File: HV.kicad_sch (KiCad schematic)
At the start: 15 parts, among them J401 1935161, J402 Header_Male_Pin_2.54mm_1X3_,_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, J403 RF1-01K-D-00-50-BK-HDW, J404 1935161, J405 RF1-01K-D-00-50-BK-HDW, Q401 MCB90N12A-TP, Q402 MCB90N12A-TP, U401 TMCS1108A4UQDR

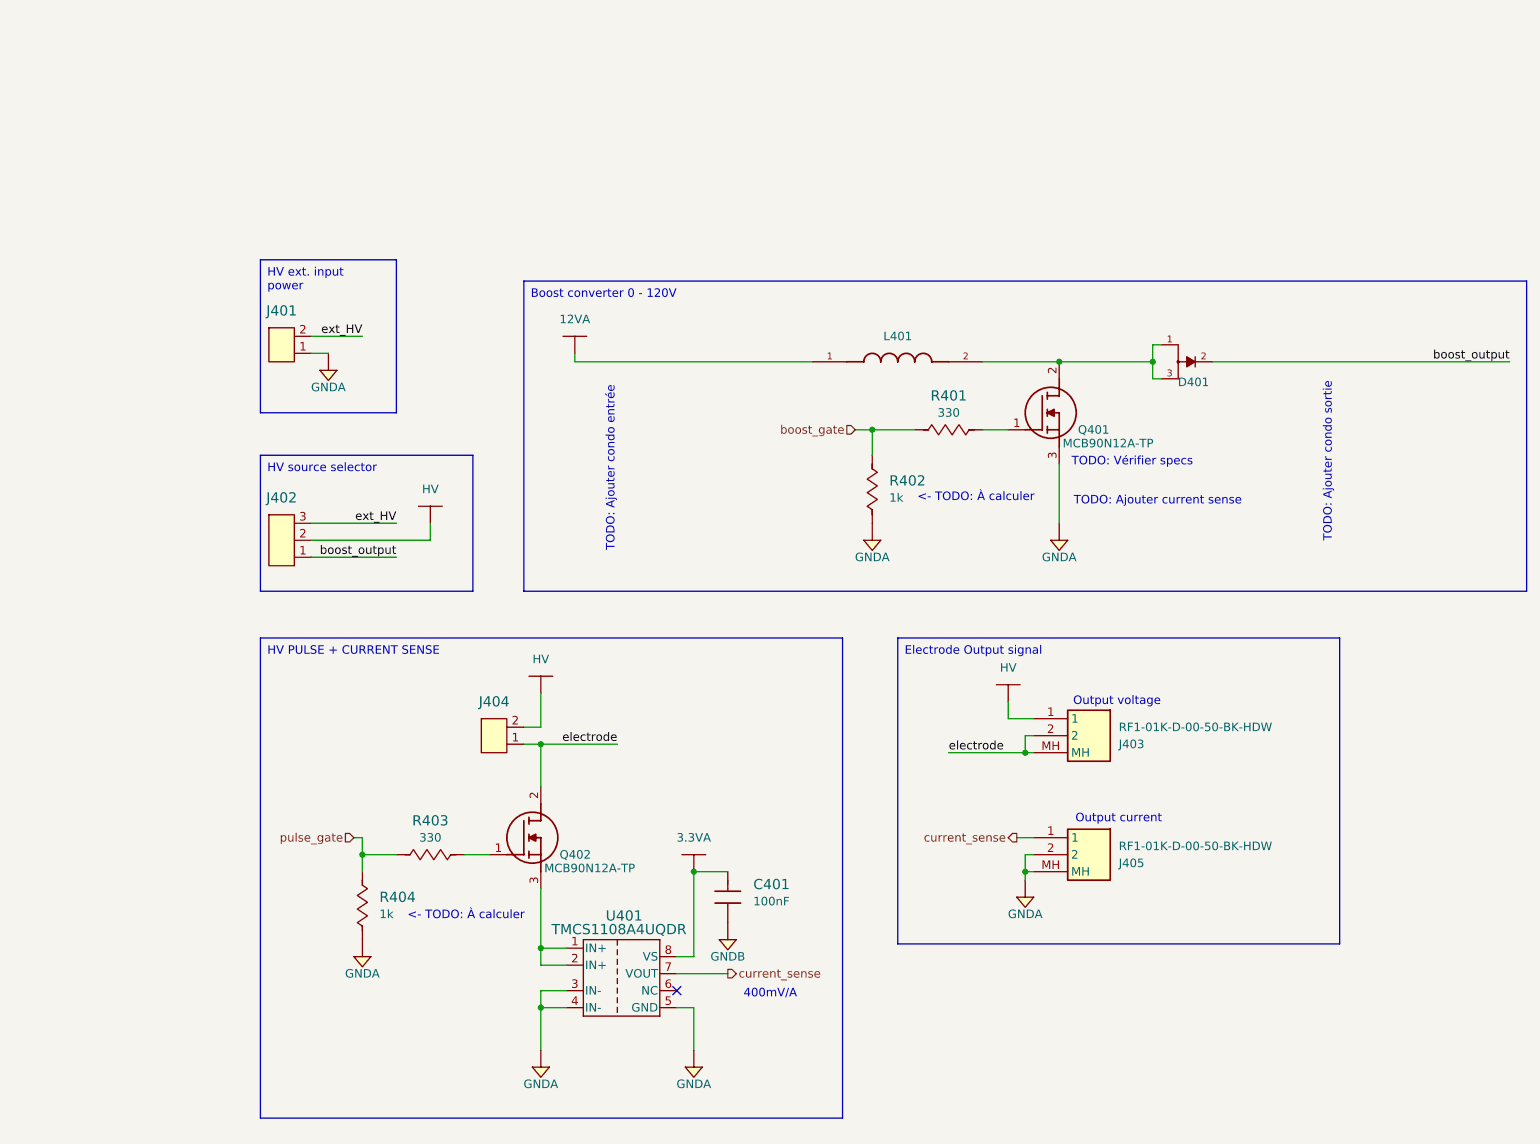
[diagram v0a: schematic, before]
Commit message: modif schématique
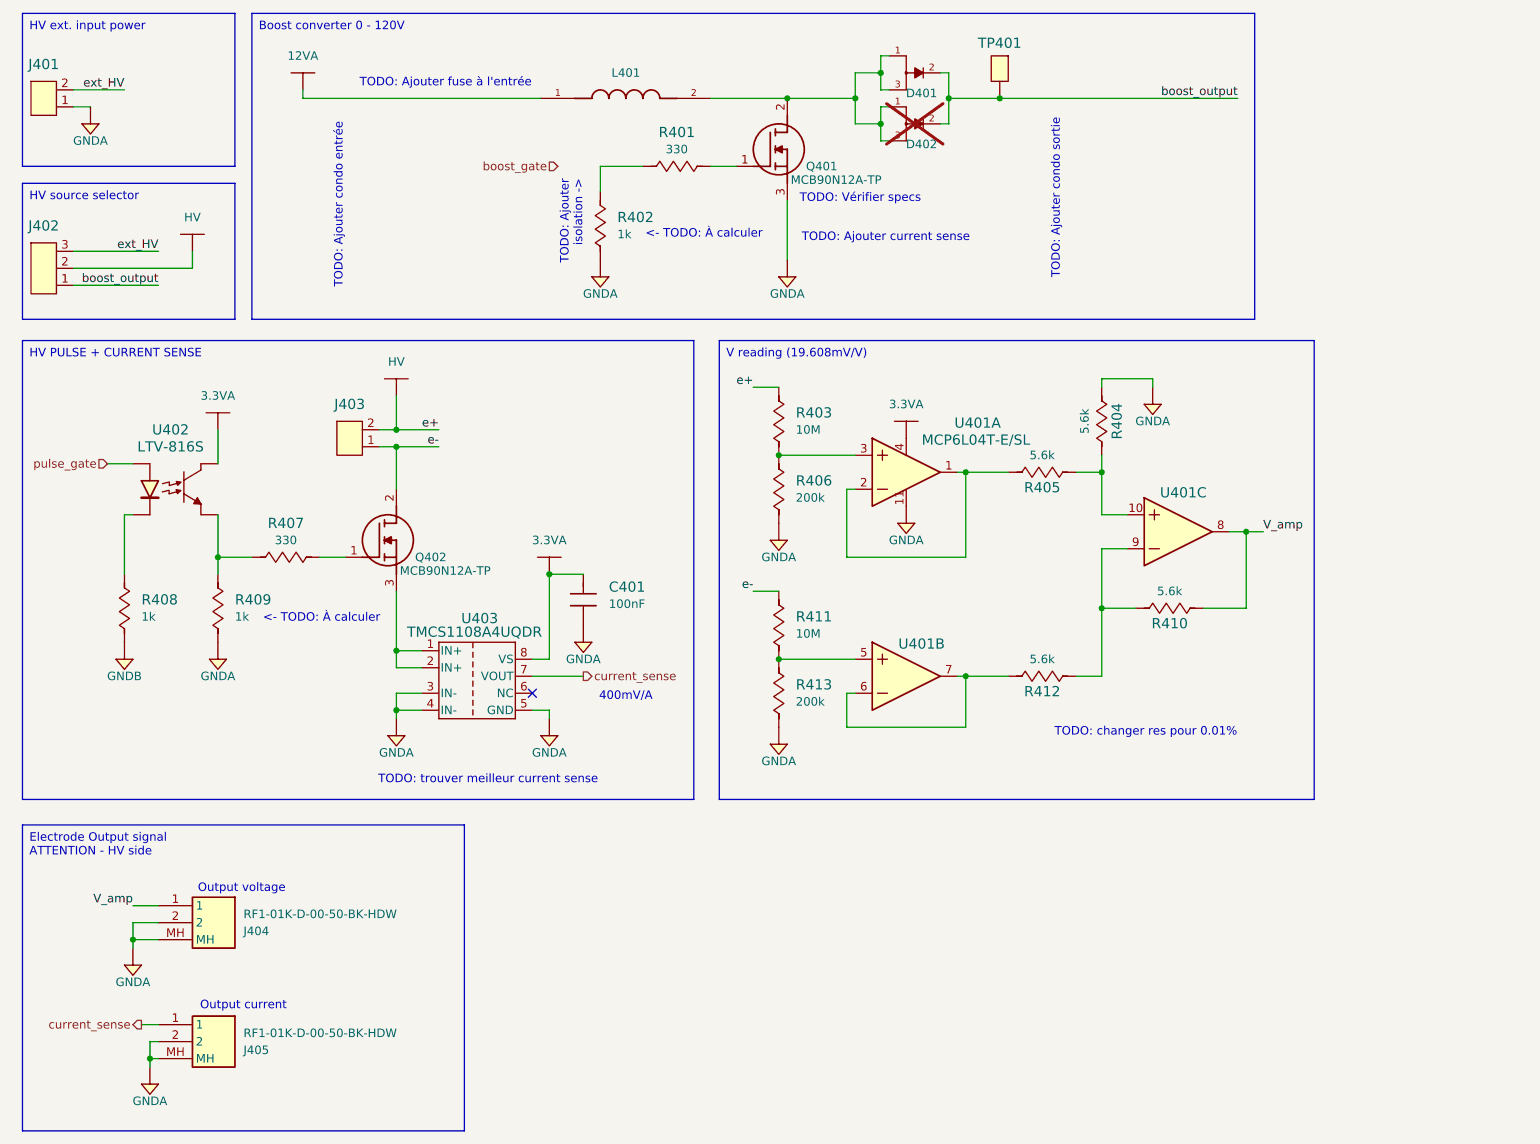
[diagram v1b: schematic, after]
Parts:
- added D401: SBRD10200TR, Diodes:DPAK228P1005X240-4N, symbol Diodes:SBRD10200TR
- added R403, R411: RMCF0805FT10M0, Resistors:R0805, symbol Resistors:RMCF0805FT10M0
- added R404, R405, R410, R412: RC0805FR-075K6L, Resistors:R0805, symbol Resistors:RC0805FR-075K6L
- added R406, R413: RC0805FR-07200KL, Resistors:R0805, symbol Resistors:RC0805FR-07200KL
- added R408: RC0805JR-071KL, Resistors:R0805, symbol Resistors:RC0805JR-071KL
- added TP401: Test_Point_THM, Connectors:Keystone_5001, symbol Connectors:Test_Point_THM
- added U401: MCP6L04T-E/SL, IC:SOIC127P600X175-14N, symbol Amplifiers:MCP6L04T-E/SL
- added U402: LTV-816S, IC:4-SMD, symbol Isolators:LTV-816S
- D402: renamed from D401; now not fitted
- renumbered J404 to J403, J403 to J404, R403 to R407, R404 to R409, U401 to U403
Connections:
- net 3.3VA: now also U401.4, U402.4 (C)
- net GNDA: now also C401.1, J404.2, J404.MH, R404.2, R406.1, R413.1, U401.11
- net GNDB: now also R408.1; no longer C401.1
- net HV: now also R403.2; no longer J404.1
- net boost_gate: no longer R401.1, R402.2
- net boost_output: now also D401.2, TP401.1 (TP)
- net pulse_gate: now also U402.1 (Anode); no longer R407.1, R409.2
- net at D402.1, D402.3, L401.2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: now also D401.1, D401.3
- net electrode renamed e-
- net e-: now also R411.2; no longer J404.2, J404.MH
- new net: R408.2, U402.2 (Cathode)
- new net: R407.1, R409.2, U402.3 (E)
- new net: R405.1, U401.1, U401.2
- new net: R404.1, R405.2, U401.10
- new net: R411.1, R413.2, U401.5
- new net: R412.1, U401.6, U401.7
- new net: R403.1, R406.2, U401.3
- new net: R401.1, R402.2
- new net: R410.1, R412.2, U401.9
- new net V_amp: J404.1, R410.2, U401.8
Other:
- note added: "TODO: Ajouter fuse à l'entrée"
- note added: "TODO: Ajouter isolation ->"
- note added: "TODO: changer res pour 0.01%"
- note added: "TODO: trouver meilleur current sense"
- moved on the sheet: C401, J401, J402, J403, J404, J405, L401, Q401, Q402, R401, R402, R407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
